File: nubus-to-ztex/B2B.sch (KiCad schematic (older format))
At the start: 13 parts, among them J1 87832-1420 (2x7 M 2mm), J3 Conn_01x06_Male

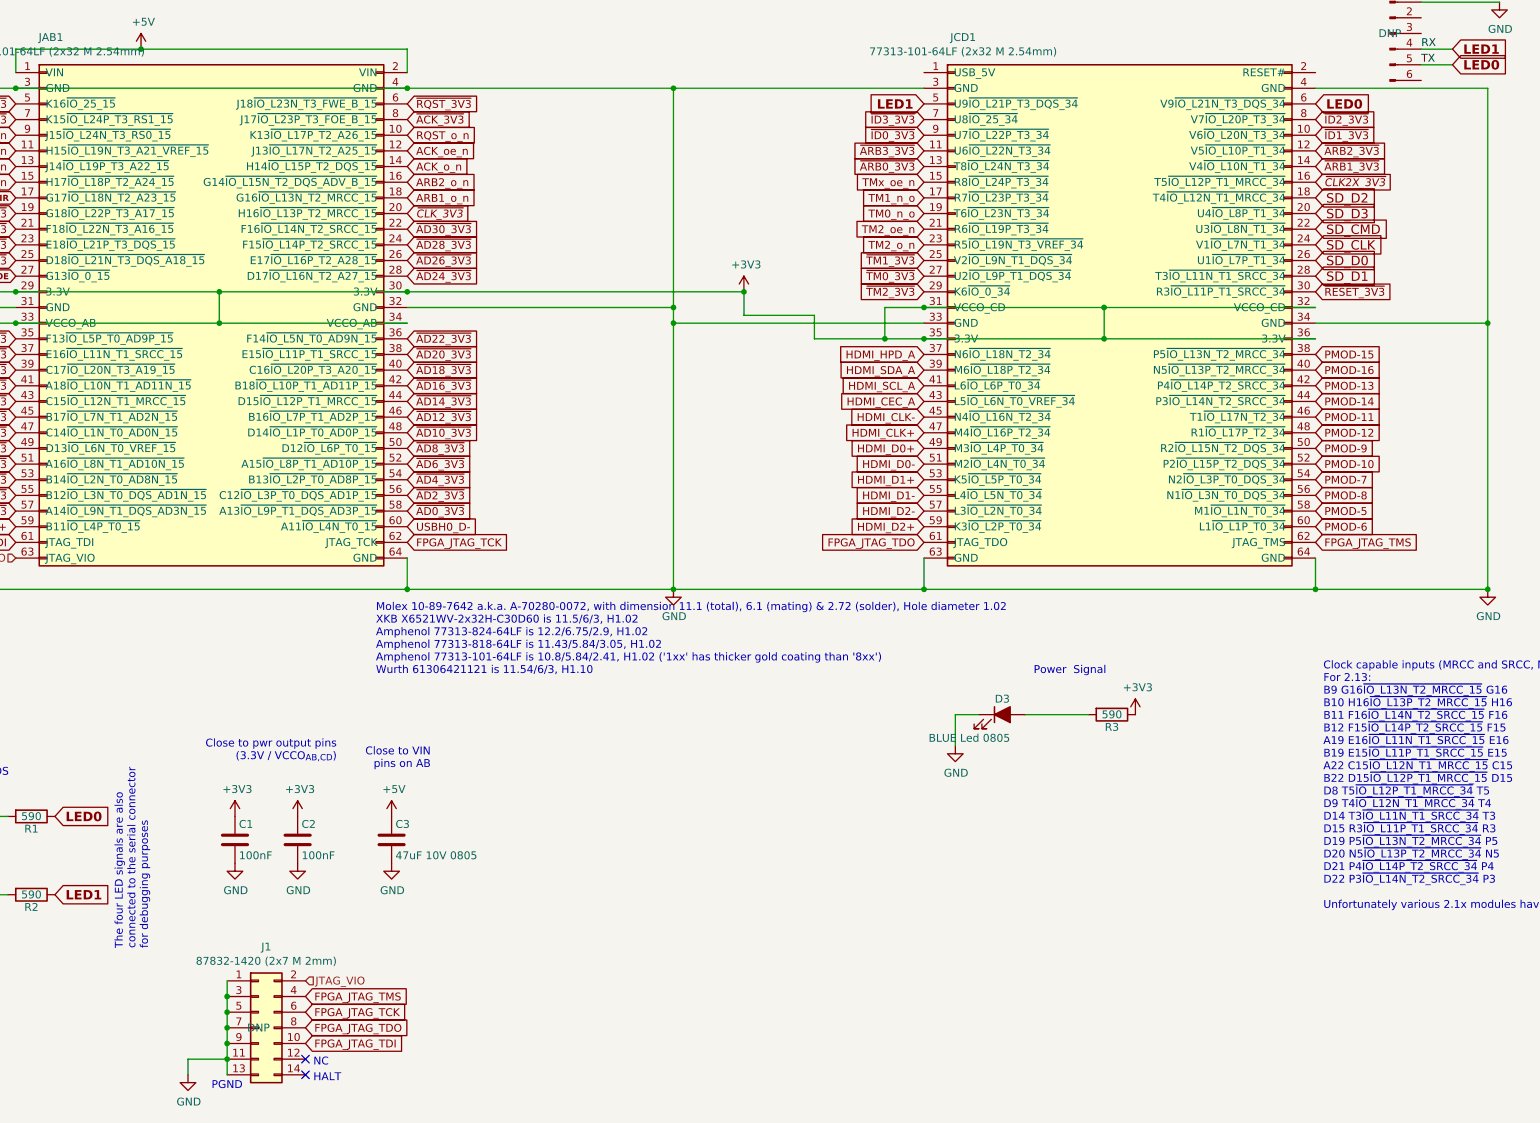
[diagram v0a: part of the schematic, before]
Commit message: update
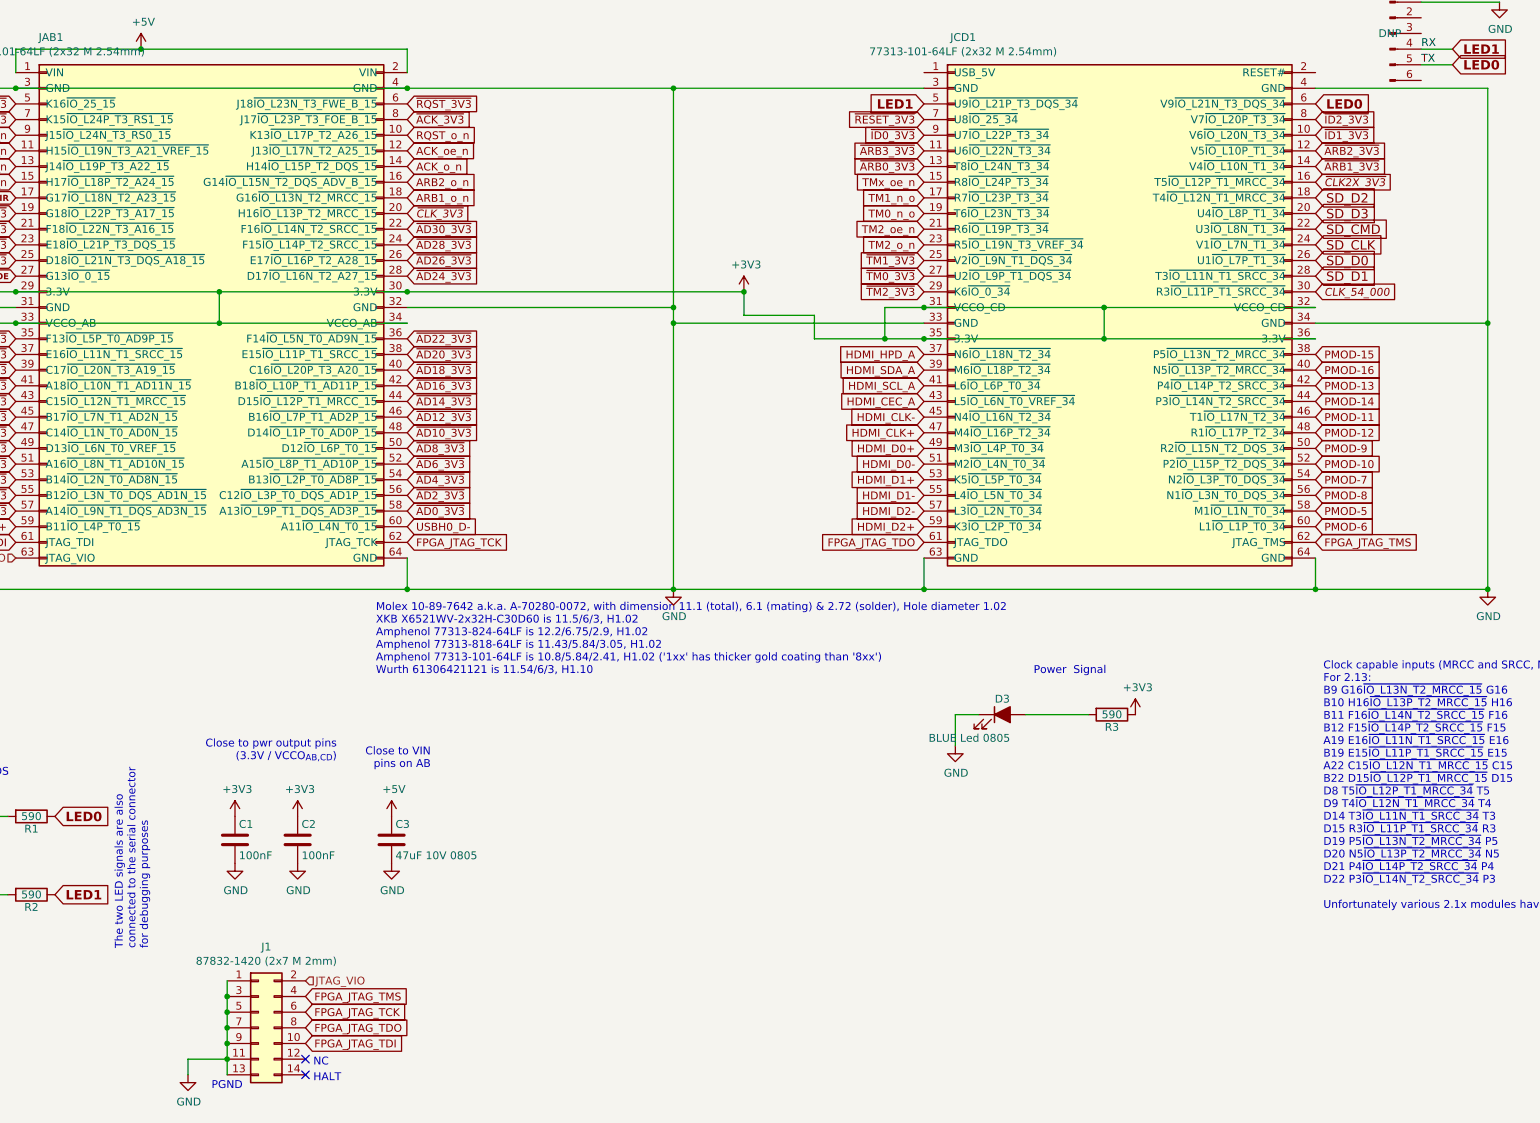
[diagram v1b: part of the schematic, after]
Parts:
- J1: DNP DNP -> (none)
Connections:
- net ~ID3_3V3 is gone; now on net ~RESET_3V3: JCD1.7 (U8~IO_25_34)
- net ~RESET_3V3: no longer JCD1.30 (R3~IO_L11P_T1_SRCC_34)
- new net CLK_54_000: JCD1.30 (R3~IO_L11P_T1_SRCC_34)
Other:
- note added: "The two LED signals are also\nconnected to the serial connector\nfor debugging purposes"
- note removed: "The four LED signals are also\nconnected to the serial connector\nfor debugging purposes"
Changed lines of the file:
@@
 $Descr A4 11693 8268
 encoding utf-8
-Sheet 2 8
+Sheet 2 9
 Title "nubus-to-ztex B2B connector"
 Date ""
@@
 F 4 "87832-1420" H 3150 7250 50  0001 C CNN "MPN"
 F 5 "https://www.mouser.fr/ProductDetail/Molex/87832-1420?qs=9Wl4wMk6Njp2JciwISLQUQ%3D%3D" H 3150 7250 50  0001 C CNN "URL"
-F 6 "DNP" H 3150 7250 50  0000 C CNN "DNP"
 	1    3150 7250
 	1    0    0    -1
@@
 Text GLabel 4100 2150 2    50   Input ~ 0
 ~AD30_3V3
-Text GLabel 9900 2550 2    50   Input ~ 0
+Text GLabel 7400 1450 0    50   Input ~ 0
 ~RESET_3V3
 Text GLabel 7400 2350 0    50   Input ~ 0
@@
 Text GLabel 7400 1550 0    50   Input ~ 0
 ~ID0_3V3
-Text GLabel 7400 1450 0    50   Input ~ 0
-~ID3_3V3
 Text GLabel 7400 3450 0    50   Input ~ 0
 HDMI_CLK+
@@
 Molex 10-89-7642 a.k.a. A-70280-0072, with dimension 11.1 (total), 6.1 (mating) & 2.72 (solder), Hole diameter 1.02\nXKB X6521WV-2x32H-C30D60 is 11.5/6/3, H1.02\nAmphenol 77313-824-64LF is 12.2/6.75/2.9, H1.02\nAmphenol 77313-818-64LF is 11.43/5.84/3.05, H1.02\nAmphenol 77313-101-64LF is 10.8/5.84/2.41, H1.02 ('1xx' has thicker gold coating than '8xx')\nWurth 61306421121 is 11.54/6/3, H1.10\n
 Text Notes 2450 6750 1    50   ~ 0
-The four LED signals are also\nconnected to the serial connector\nfor debugging purposes
+The two LED signals are also\nconnected to the serial connector\nfor debugging purposes
 Connection ~ 6250 2550
 Text GLabel 9900 3250 2    50   Input ~ 0
@@
 Wire Wire Line
 	10575 1100 10775 1100
+Text GLabel 9900 2550 2    50   Input Italic 0
+CLK_54_000
 $EndSCHEMATC
